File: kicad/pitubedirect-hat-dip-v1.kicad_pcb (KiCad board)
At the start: 2 copper layers, 58.4 x 63.5 mm, 25 parts, among them P1 CONN_02X20, P2 CONN_02X13, P3 CONN_01X02, P4 CONN_01X03, U1 74LVC245AN, U2 74LVC245AN

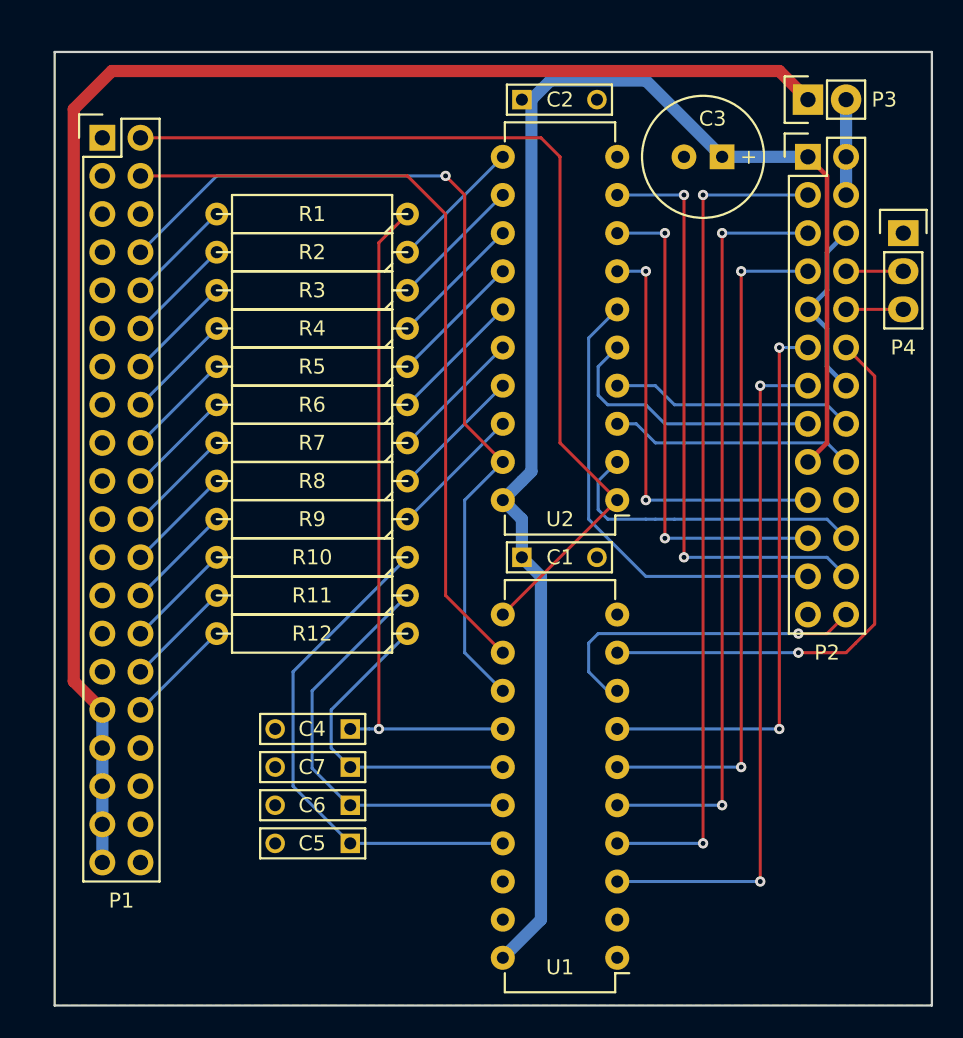
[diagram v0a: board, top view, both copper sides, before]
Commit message: Added 2nd iteration of PCB design
Change-Id: I13e39ce9abf2ba7743cdcd9543cd2f85d4fc066c
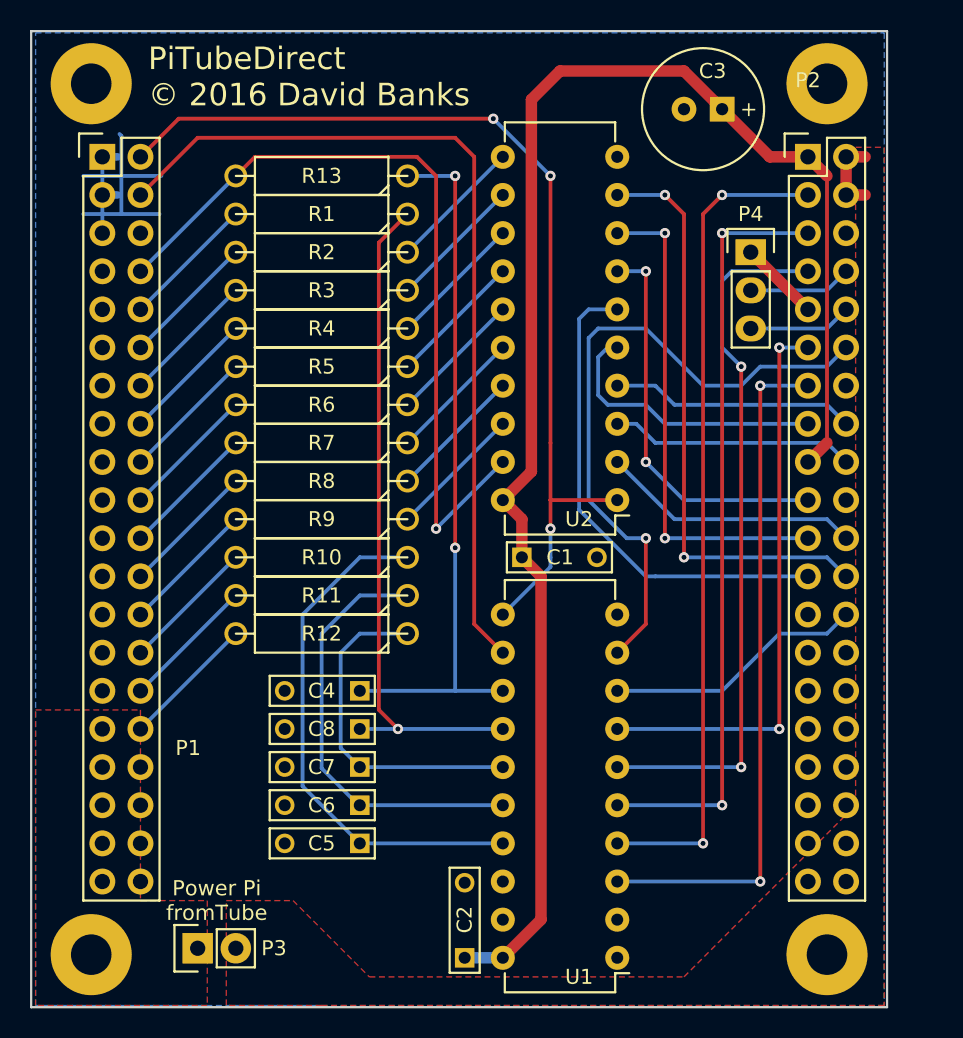
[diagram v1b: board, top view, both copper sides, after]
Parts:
- added C8: 15p, Capacitors_ThroughHole:C_Rect_L7_W2_P5, F.Cu at (138.4, 113.7)
- added R13: 470, Discret:R4-5, F.Cu at (135.9, 79.4)
- added REF**: MountingHole_2.7mm_M2.5_Pad, Mounting_Holes:MountingHole_2.7mm_M2.5_Pad, F.Cu at (169.5, 73.2)
- added REF**: MountingHole_2.7mm_M2.5_Pad, Mounting_Holes:MountingHole_2.7mm_M2.5_Pad, F.Cu at (169.5, 131.2)
- added REF**: MountingHole_2.7mm_M2.5_Pad, Mounting_Holes:MountingHole_2.7mm_M2.5_Pad, F.Cu at (120.5, 73.2)
- added REF**: MountingHole_2.7mm_M2.5_Pad, Mounting_Holes:MountingHole_2.7mm_M2.5_Pad, F.Cu at (120.5, 131.2)
- P2: value CONN_02X13 -> CONN_02X20; footprint Pin_Headers:Pin_Header_Straight_2x13 -> Pin_Headers:Pin_Header_Straight_2x20
- R1, R10, R11, R12, R2, R3, R4, R5, R6, R7, R8, R9: footprint Discret:R5 -> Discret:R4-5
- moved P3 69.6 mm to (127.6, 130.8)
- moved C2 57.3 mm to (145.4, 131.4), turned to 90 degrees
- moved P4 10.2 mm to (164.5, 84.5)
- moved C3 3.17 mm to (161.3, 74.9)
- moved P1 1.27 mm to (121.3, 78.1)
- moved C4 0.64 mm to (138.4, 116.2)
- moved C5 0.64 mm to (138.4, 123.8)
- moved C6 0.64 mm to (138.4, 121.3)
- moved C7 0.64 mm to (138.4, 118.7)
- moved R1 0.63 mm to (135.9, 81.9)
- moved R10 0.63 mm to (135.9, 104.8)
- moved R11 0.63 mm to (135.9, 107.3)
- moved R12 0.63 mm to (135.9, 109.9)
- moved R2 0.63 mm to (135.9, 84.5)
- moved R3 0.63 mm to (135.9, 87.0)
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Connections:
- P1 pad 8: /TnTUBE -> Net-(P1-Pad8)
- U2 pad 19: /TnTUBE -> Net-(P1-Pad8)
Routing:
- net +5V: track 101.7 -> 0.00 mm
- net Net-(P1-Pad8): track 0.00 -> 53.1 mm, vias 0 -> 1
- net GND: track 12.3 -> 28.3 mm
- net /TnTUBE: track 60.4 -> 47.0 mm, vias 1 -> 2
- net /RnW: track 37.1 -> 44.7 mm
- net /TPHI2: track 52.2 -> 58.1 mm
- net /PHI2: track 22.3 -> 18.0 mm, vias 1 -> 0
- net /D7: track 21.0 -> 17.3 mm
- net VCC: track 102.5 -> 105.5 mm
- net Net-(P2-Pad8): track 3.81 -> 6.88 mm
- net Net-(P2-Pad10): track 3.81 -> 6.88 mm
- net /TRnW: track 63.7 -> 65.5 mm, vias 0 -> 3
- net Net-(P1-Pad30): track 7.18 -> 8.98 mm
- net Net-(P1-Pad20): track 7.18 -> 8.98 mm
- net Net-(P1-Pad16): track 7.18 -> 8.98 mm
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- added copper zone on F.Cu, net +5V
- added copper zone on F.Cu, net Net-(P2-Pad2)
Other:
- board size 58.4 x 63.5 mm -> 57 x 65 mm
- net class Default: clearance 0.2032 -> 0.254; trace_width 0.2032 -> 0.254
- net class Power: clearance 0.2032 -> 0.254; trace_width 0.3048 -> 0.762
- rule trace_clearance: 0.2032 -> 0.254
- rule trace_min: 0.2032 -> 0.254
- board text added: "PiTubeDirect © 2016 David Banks"
- board text added: "Power Pi fromTube"
